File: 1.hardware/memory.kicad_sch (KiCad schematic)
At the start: 71 parts, among them IC2 IS42S32800J-6TLI, U6 W25Q128JVS, U7 NC_IS42S16400J-xC

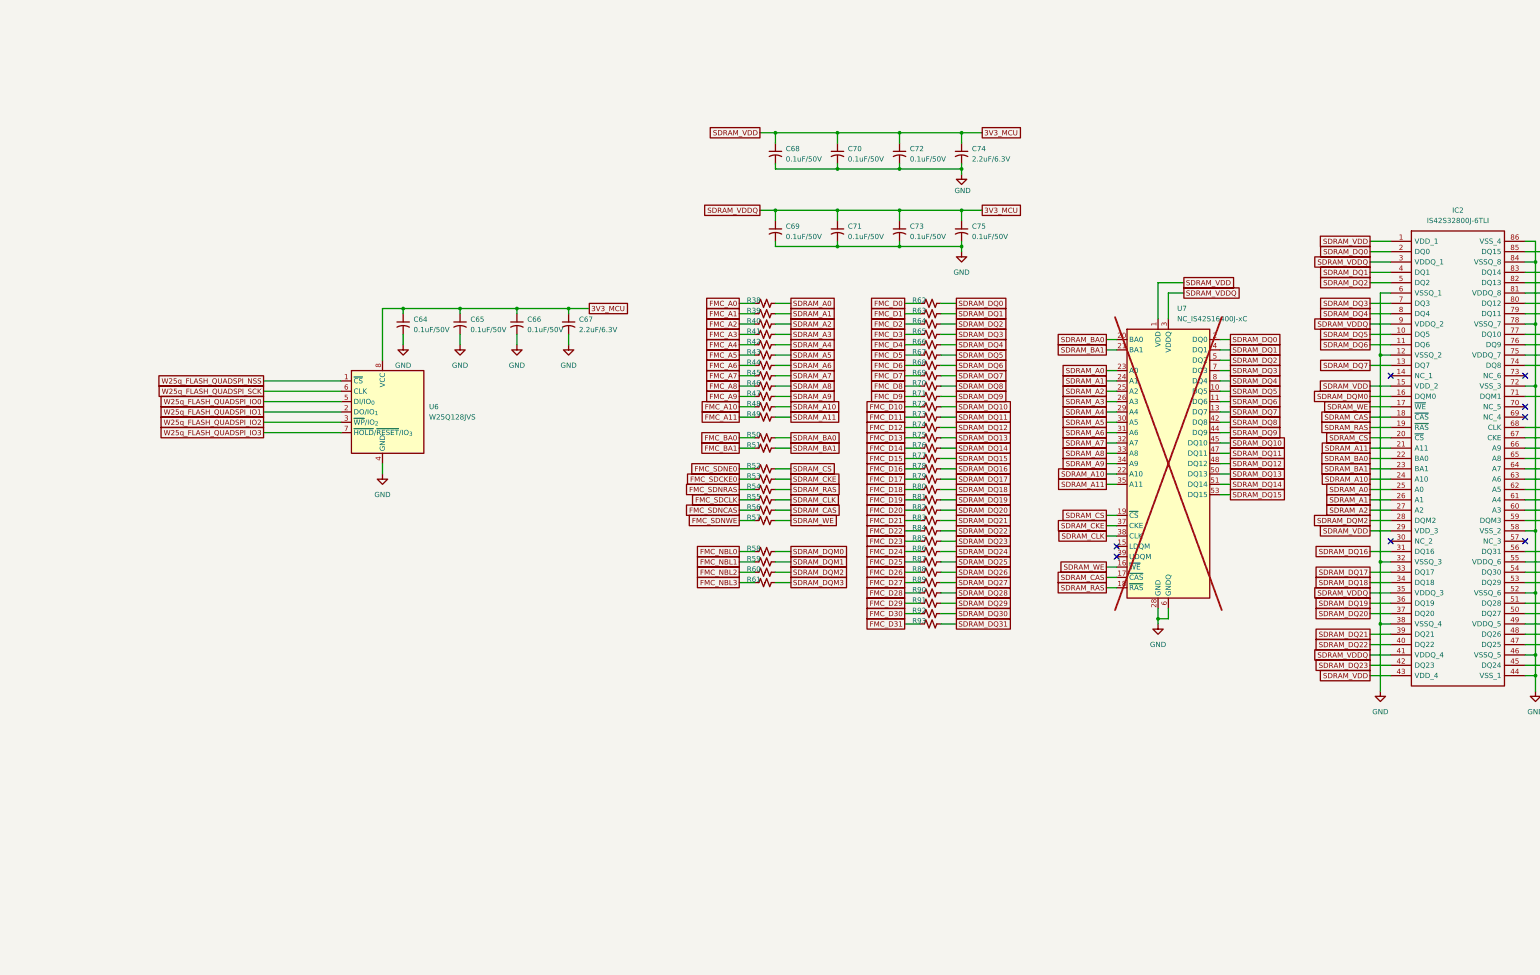
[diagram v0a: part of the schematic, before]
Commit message: 중간 저장
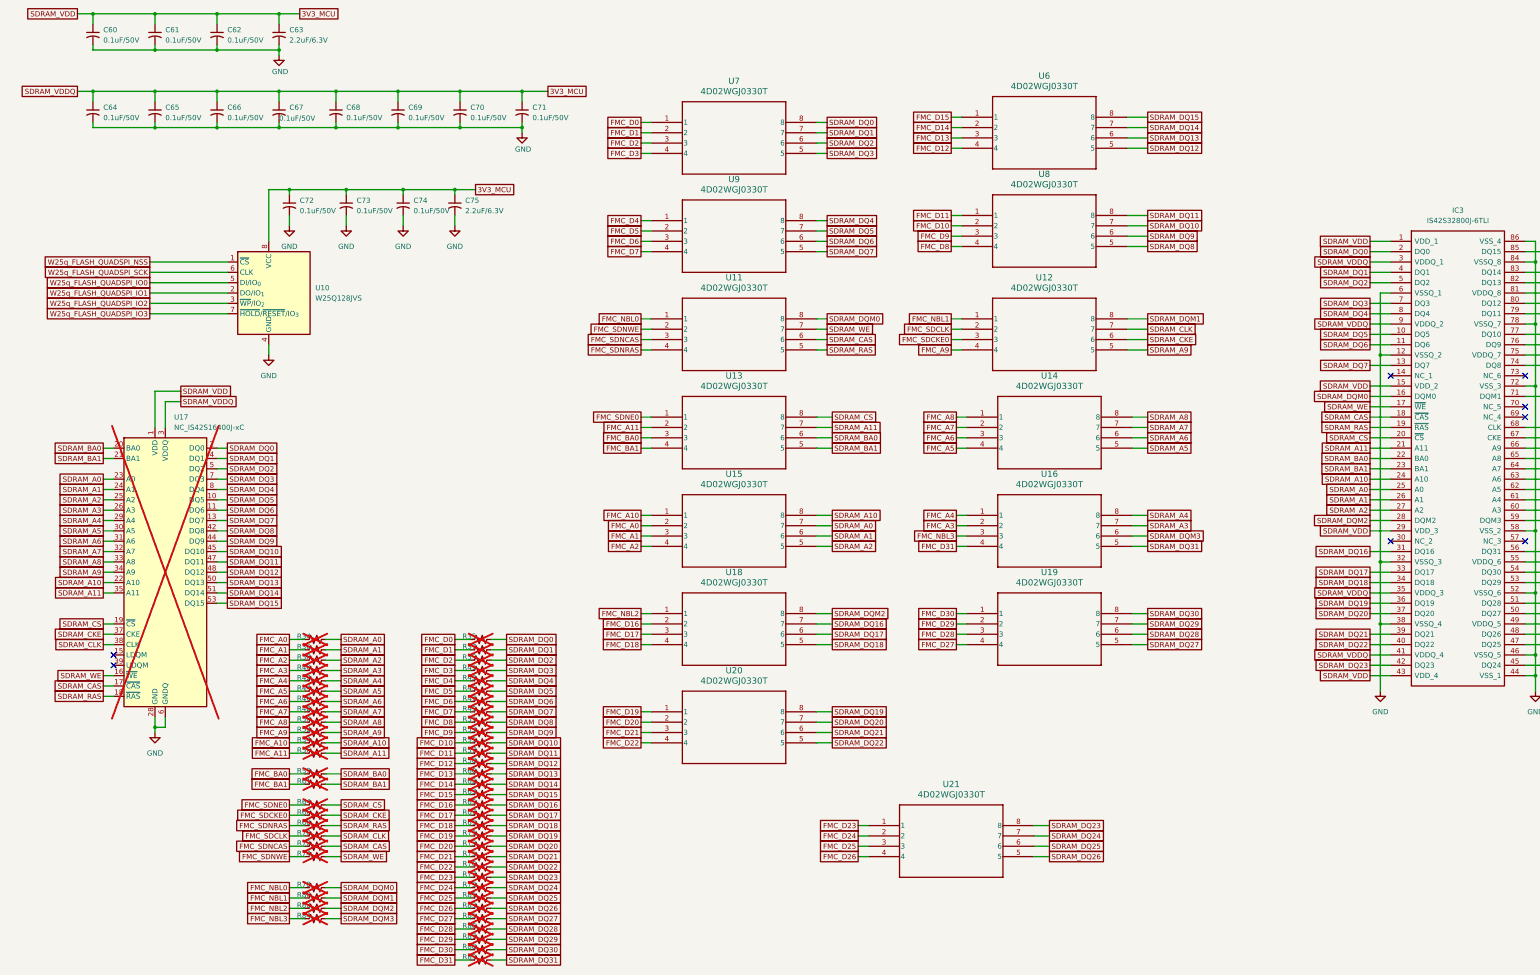
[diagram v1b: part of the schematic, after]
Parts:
- added C68, C69, C70, C71: 0.1uF/50V, Capacitor_SMD:C_0603_1608Metric, symbol Device:C_Small_US
- added U11, U12, U13, U14, U15, U16, U18, U19, U20, U21, U6, U7, U8, U9: 4D02WGJ0330T, 4D02_2X1_ROH, symbol 2025-12-16_06-00-56:4D02WGJ0330T
- R34: renamed from R38; now not fitted; now left out of the parts list
- R35: renamed from R62; now not fitted; now left out of the parts list
- R36: renamed from R39; now not fitted; now left out of the parts list
- R37: renamed from R63; now not fitted; now left out of the parts list
- R38: renamed from R40; now not fitted; now left out of the parts list
- R39: renamed from R64; now not fitted; now left out of the parts list
- R40: renamed from R41; now not fitted; now left out of the parts list
- R41: renamed from R65; now not fitted; now left out of the parts list
- R42: now not fitted; now left out of the parts list
- R43: renamed from R66; now not fitted; now left out of the parts list
- R44: renamed from R43; now not fitted; now left out of the parts list
- R45: renamed from R67; now not fitted; now left out of the parts list
- R46: renamed from R44; now not fitted; now left out of the parts list
- R47: renamed from R68; now not fitted; now left out of the parts list
- R48: renamed from R45; now not fitted; now left out of the parts list
- R49: renamed from R69; now not fitted; now left out of the parts list
- R50: renamed from R46; now not fitted; now left out of the parts list
- R51: renamed from R70; now not fitted; now left out of the parts list
- R52: renamed from R47; now not fitted; now left out of the parts list
- R53: renamed from R71; now not fitted; now left out of the parts list
- R54: renamed from R48; now not fitted; now left out of the parts list
- R55: renamed from R72; now not fitted; now left out of the parts list
- R56: renamed from R49; now not fitted; now left out of the parts list
- R57: renamed from R73; now not fitted; now left out of the parts list
- R58: renamed from R74; now not fitted; now left out of the parts list
- R59: renamed from R50; now not fitted; now left out of the parts list
- R60: renamed from R75; now not fitted; now left out of the parts list
- R61: renamed from R51; now not fitted; now left out of the parts list
- R62: renamed from R76; now not fitted; now left out of the parts list
- R63: renamed from R77; now not fitted; now left out of the parts list
- R64: renamed from R52; now not fitted; now left out of the parts list
- R65: renamed from R78; now not fitted; now left out of the parts list
- R66: renamed from R53; now not fitted; now left out of the parts list
- R67: renamed from R79; now not fitted; now left out of the parts list
- R68: renamed from R54; now not fitted; now left out of the parts list
- R69: renamed from R80; now not fitted; now left out of the parts list
- R70: renamed from R55; now not fitted; now left out of the parts list
- R71: renamed from R81; now not fitted; now left out of the parts list
- R72: renamed from R56; now not fitted; now left out of the parts list
- R73: renamed from R82; now not fitted; now left out of the parts list
- R74: renamed from R57; now not fitted; now left out of the parts list
- R75: renamed from R83; now not fitted; now left out of the parts list
- R76: renamed from R84; now not fitted; now left out of the parts list
- R77: renamed from R85; now not fitted; now left out of the parts list
- R78: renamed from R58; now not fitted; now left out of the parts list
- R79: renamed from R86; now not fitted; now left out of the parts list
- R80: renamed from R59; now not fitted; now left out of the parts list
- R81: renamed from R87; now not fitted; now left out of the parts list
- R82: renamed from R60; now not fitted; now left out of the parts list
- R83: renamed from R88; now not fitted; now left out of the parts list
- R84: renamed from R61; now not fitted; now left out of the parts list
- R85: renamed from R89; now not fitted; now left out of the parts list
- R86: renamed from R90; now not fitted; now left out of the parts list
- R87: renamed from R91; now not fitted; now left out of the parts list
- R88: renamed from R92; now not fitted; now left out of the parts list
- R89: renamed from R93; now not fitted; now left out of the parts list
- renumbered C68 to C60, C70 to C61, C72 to C62, C74 to C63, C69 to C64, C71 to C65, C73 to C66, C75 to C67, C64 to C72, C65 to C73, C66 to C74, C67 to C75, IC2 to IC3, U6 to U10, U7 to U17
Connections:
- net 3V3_MCU: now also C68.1, C69.1, C70.1, C71.1
- net FMC_A0: now also U15.2
- net FMC_A1: now also U15.3
- net FMC_A10: now also U15.1
- net FMC_A11: now also U13.2
- net FMC_A2: now also U15.4
- net FMC_A3: now also U16.2
- net FMC_A4: now also U16.1
- net FMC_A5: now also U14.4
- net FMC_A6: now also U14.3
- net FMC_A7: now also U14.2
- net FMC_A8: now also U14.1
- net FMC_A9: now also U12.4
- net FMC_BA0: now also U13.3
- net FMC_BA1: now also U13.4
- net FMC_D0: now also U7.1
- net FMC_D1: now also U7.2
- net FMC_D10: now also U8.2
- net FMC_D11: now also U8.1
- net FMC_D12: now also U6.4
- net FMC_D13: now also U6.3
- net FMC_D14: now also U6.2
- net FMC_D15: now also U6.1
- net FMC_D16: now also U18.2
- net FMC_D17: now also U18.3
- net FMC_D18: now also U18.4
- net FMC_D19: now also U20.1
- net FMC_D2: now also U7.3
- net FMC_D20: now also U20.2
- net FMC_D21: now also U20.3
- net FMC_D22: now also U20.4
- net FMC_D23: now also U21.1
- net FMC_D24: now also U21.2
- net FMC_D25: now also U21.3
- net FMC_D26: now also U21.4
- net FMC_D27: now also U19.4
- net FMC_D28: now also U19.3
- net FMC_D29: now also U19.2
- net FMC_D3: now also U7.4
- net FMC_D30: now also U19.1
- net FMC_D31: now also U16.4
- net FMC_D4: now also U9.1
- net FMC_D5: now also U9.2
- net FMC_D6: now also U9.3
- net FMC_D7: now also U9.4
- net FMC_D8: now also U8.4
- net FMC_D9: now also U8.3
- net FMC_NBL0: now also U11.1
- net FMC_NBL1: now also U12.1
- net FMC_NBL2: now also U18.1
- net FMC_NBL3: now also U16.3
- net FMC_SDCKE0: now also U12.3
- net FMC_SDCLK: now also U12.2
- net FMC_SDNCAS: now also U11.3
- net FMC_SDNE0: now also U13.1
- net FMC_SDNRAS: now also U11.4
- net FMC_SDNWE: now also U11.2
- net GND: now also C68.2, C69.2, C70.2, C71.2
- net SDRAM_A0: now also U15.7
- net SDRAM_A1: now also U15.6
- net SDRAM_A10: now also U15.8
- net SDRAM_A11: now also U13.7
- net SDRAM_A2: now also U15.5
- net SDRAM_A3: now also U16.7
- net SDRAM_A4: now also U16.8
- net SDRAM_A5: now also U14.5
- net SDRAM_A6: now also U14.6
- net SDRAM_A7: now also U14.7
- net SDRAM_A8: now also U14.8
- net SDRAM_A9: now also U12.5
- net SDRAM_BA0: now also U13.6
- net SDRAM_BA1: now also U13.5
- net SDRAM_CAS: now also U11.6
- net SDRAM_CKE: now also U12.6
- net SDRAM_CLK: now also U12.7
- net SDRAM_CS: now also U13.8
- net SDRAM_DQ0: now also U7.8
- net SDRAM_DQ1: now also U7.7
- net SDRAM_DQ10: now also U8.7
- net SDRAM_DQ11: now also U8.8
- net SDRAM_DQ12: now also U6.5
- net SDRAM_DQ13: now also U6.6
- net SDRAM_DQ14: now also U6.7
- net SDRAM_DQ15: now also U6.8
- net SDRAM_DQ16: now also U18.7
- net SDRAM_DQ17: now also U18.6
- net SDRAM_DQ18: now also U18.5
- net SDRAM_DQ19: now also U20.8
- net SDRAM_DQ2: now also U7.6
- net SDRAM_DQ20: now also U20.7
- net SDRAM_DQ21: now also U20.6
- net SDRAM_DQ22: now also U20.5
- net SDRAM_DQ23: now also U21.8
- net SDRAM_DQ24: now also U21.7
- net SDRAM_DQ25: now also U21.6
- net SDRAM_DQ26: now also U21.5
- net SDRAM_DQ27: now also U19.5
- net SDRAM_DQ28: now also U19.6
- net SDRAM_DQ29: now also U19.7
- net SDRAM_DQ3: now also U7.5
- net SDRAM_DQ30: now also U19.8
- net SDRAM_DQ31: now also U16.5
- net SDRAM_DQ4: now also U9.8
- net SDRAM_DQ5: now also U9.7
- net SDRAM_DQ6: now also U9.6
- net SDRAM_DQ7: now also U9.5
- net SDRAM_DQ8: now also U8.5
- net SDRAM_DQ9: now also U8.6
- net SDRAM_DQM0: now also U11.8
- net SDRAM_DQM1: now also U12.8
- net SDRAM_DQM2: now also U18.8
- net SDRAM_DQM3: now also U16.6
- net SDRAM_RAS: now also U11.5
- net SDRAM_WE: now also U11.7
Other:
- moved on the sheet: C60, C61, C62, C63, C64, C65, C66, C67, C72, C73, C74, C75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
